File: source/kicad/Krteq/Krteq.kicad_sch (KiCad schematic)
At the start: 131 parts, among them J71 OLED 128x32, SW1 Switch, SW10 Switch, SW11 Switch, SW12 Switch, SW13 Switch, SW14 Switch, SW15 Switch, SW16 Switch, SW17 Switch, SW18 Switch, SW19 Switch, SW2 Switch, SW20 Switch, SW21 Switch, SW22 Switch, SW23 Switch, SW24 Switch, SW25 Switch, SW26 Switch, SW27 Switch, SW28 Switch, SW29 Switch, SW3 Switch, SW30 Switch, SW31 Switch, SW32 Switch, SW33 Switch, SW34 Switch, SW35 Switch, SW36 Switch, SW37 Switch, SW38 Switch, SW39 Switch, SW4 Switch, SW40 Switch, SW41 Switch, SW42 Switch, SW43 Switch, SW44 Switch, SW45 Switch, SW46 Switch, SW47 Switch, SW48 Switch, SW49 Switch, SW5 Switch, SW50 Switch, SW51 Switch, SW52 Switch, SW53 Switch, SW54 Switch, SW55 Switch, SW56 Switch, SW57 Switch, SW58 Switch, SW59 Switch, SW6 Switch, SW60 Switch, SW61 Switch, SW7 Switch, SW8 Switch, SW9 Switch, U71 IS31FL3733-QF

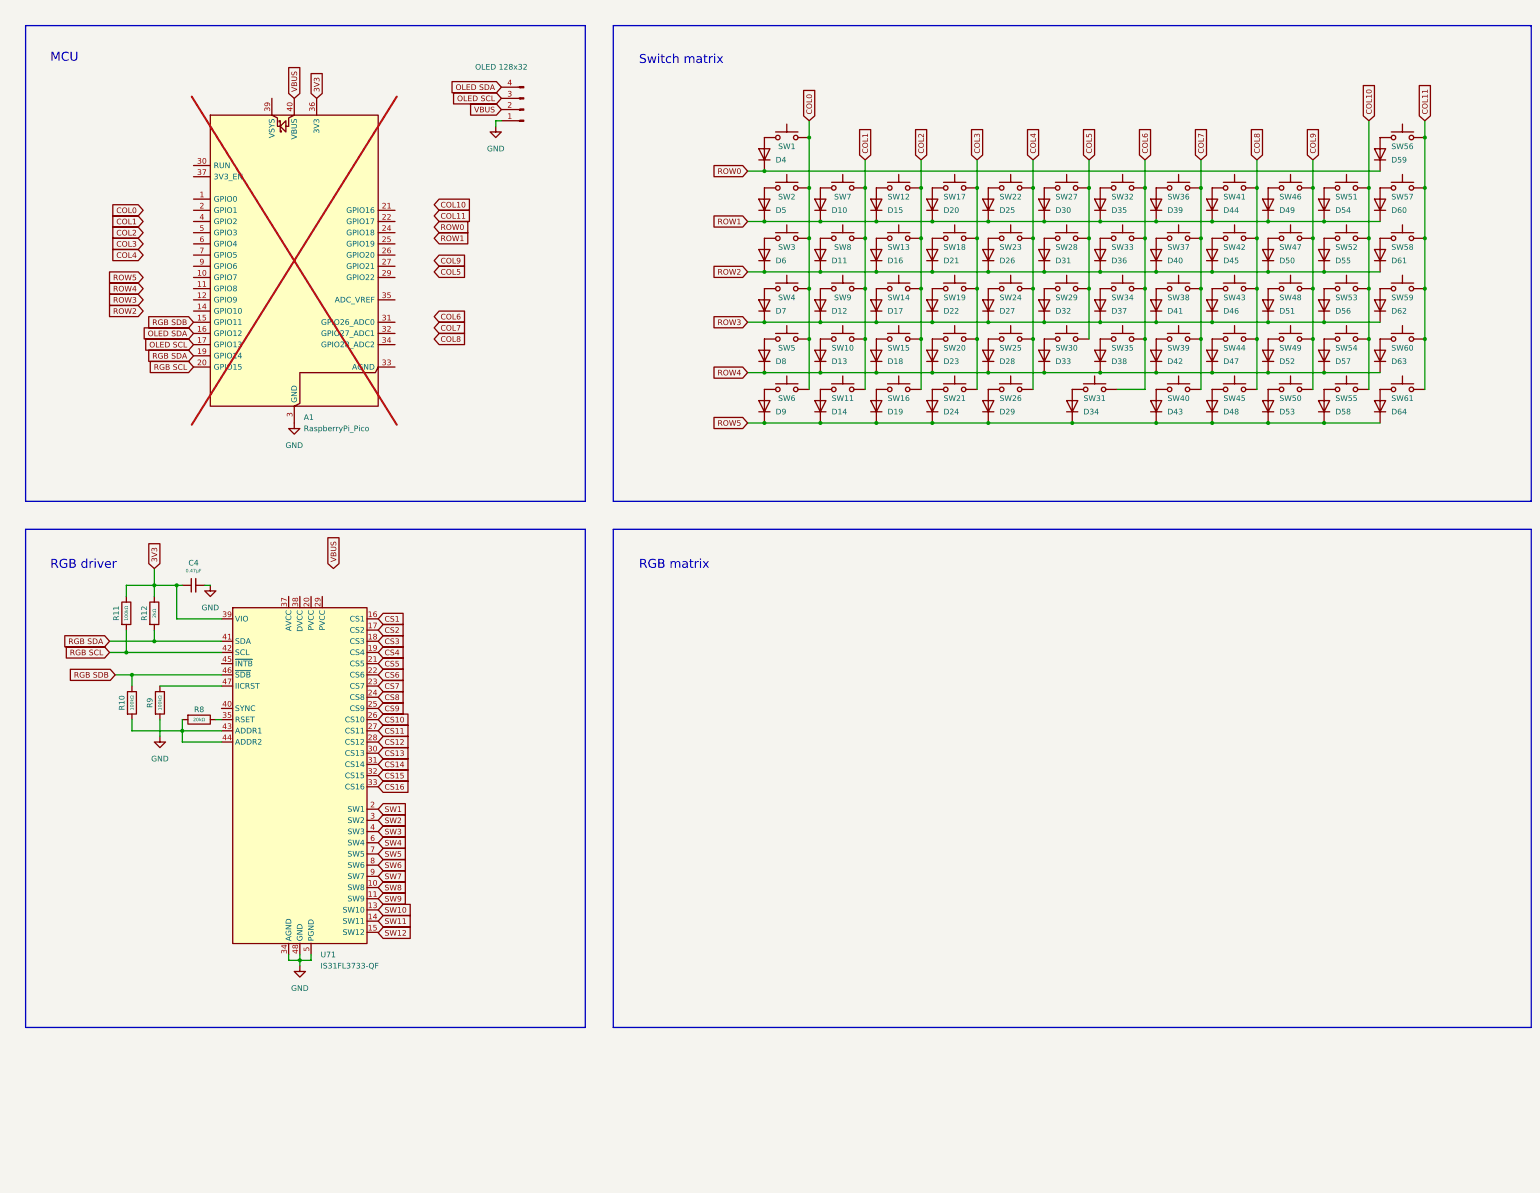
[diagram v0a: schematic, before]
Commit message: update
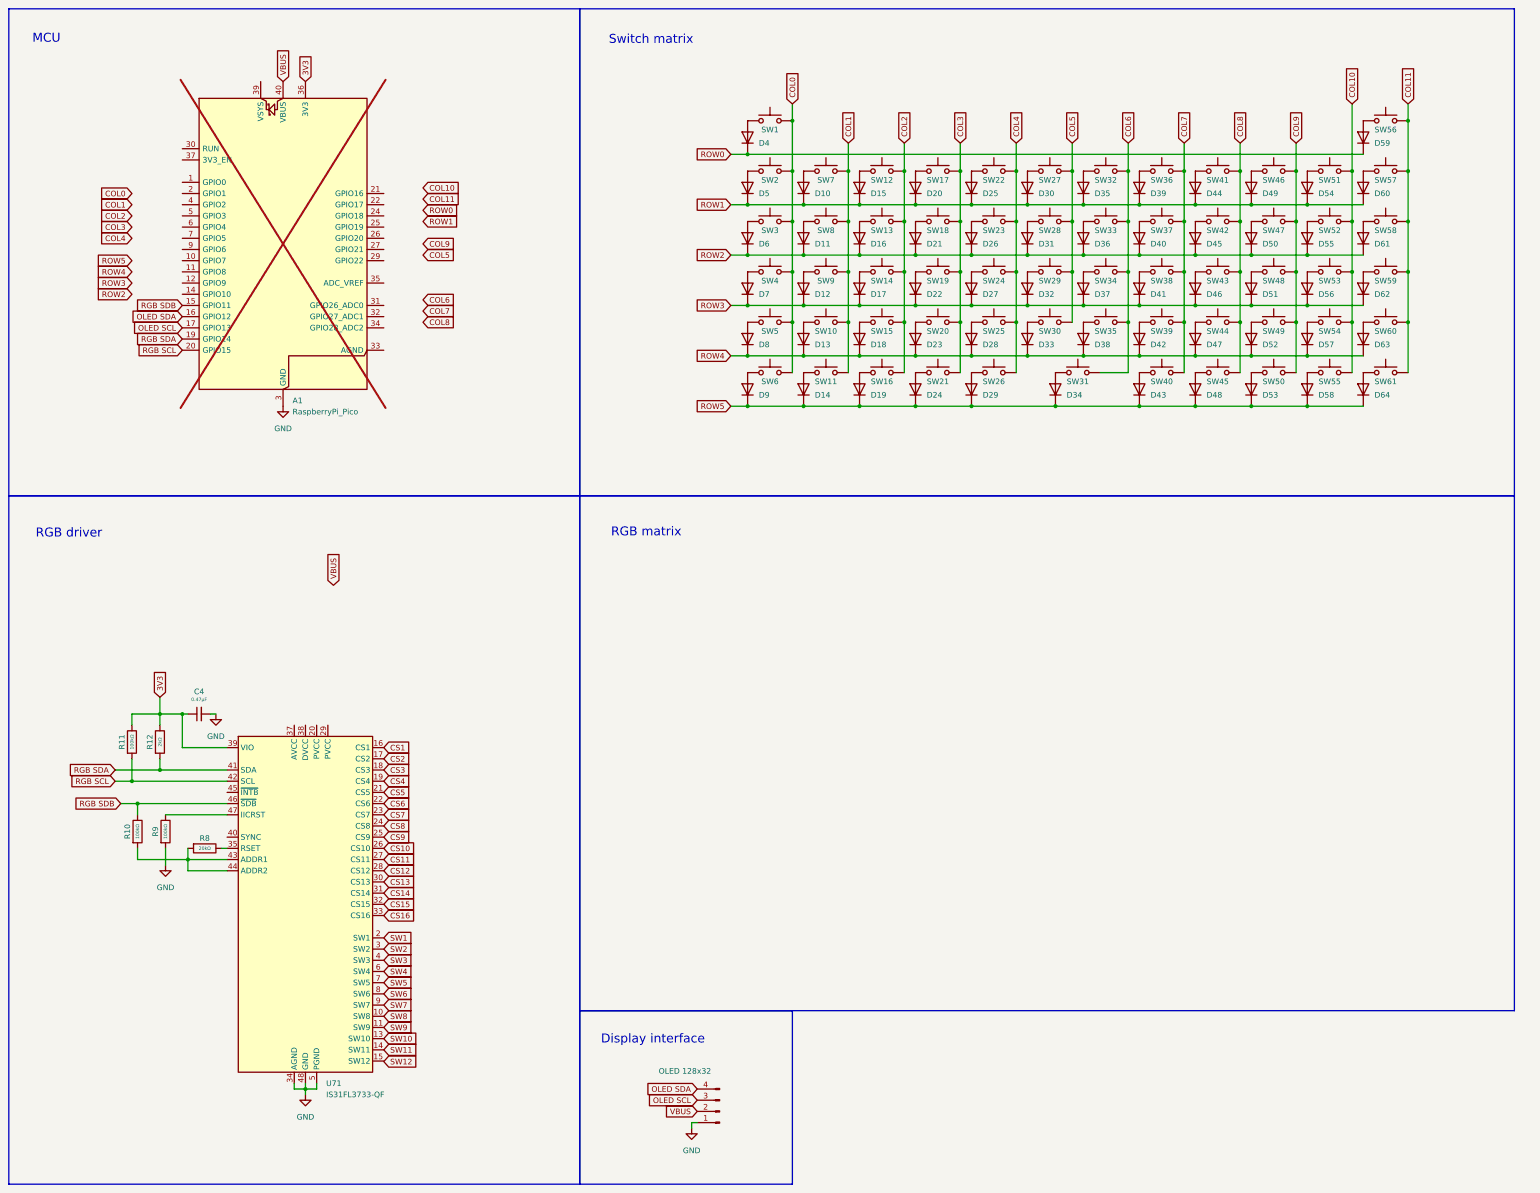
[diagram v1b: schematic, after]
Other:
- note added: "Display interface"
- moved on the sheet: A1, C4, D10, D11, D12, D13, D14, D15, D16, D17, D18, D19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
